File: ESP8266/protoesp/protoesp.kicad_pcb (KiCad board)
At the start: 2 copper layers, 97.5 x 90 mm, 192 parts, among them CN1 EPINS_TOP, CN10 USB_CURSED, CN11 CH_SPI, CN12 CH_I2C, CN13 CH341_PROG, CN14 CH_PROG, CN2 EPINS_BOTTOM, CN20 BATT, CN3 ESP_PROG, CN30 BUTTON_CONN, CN31 LDR_CONN, CN32 RGB_CONN, CN33 595_CONN, CN34 595_OUTS, CN35 595CHAIN_CONN, CN36 E_I2C, CN37 E_SPI, CN38 DRV_CONN, J1 0R, J11 0R, J17 0R, J19 0R, J2 0R, J22 0R, J7 0R, J8 0R, J9 0R, P1 PROTO_SPACE, Q1 BC817, Q2 CJ2305, SW1 RST, SW2 BUTTON, U1 CH341, U2 AP1117-33, U3 LTH7R, U4 74HC595, U5 AP2112K-3.3, U6 ESP32-WROOM-32, Y1 12MHz

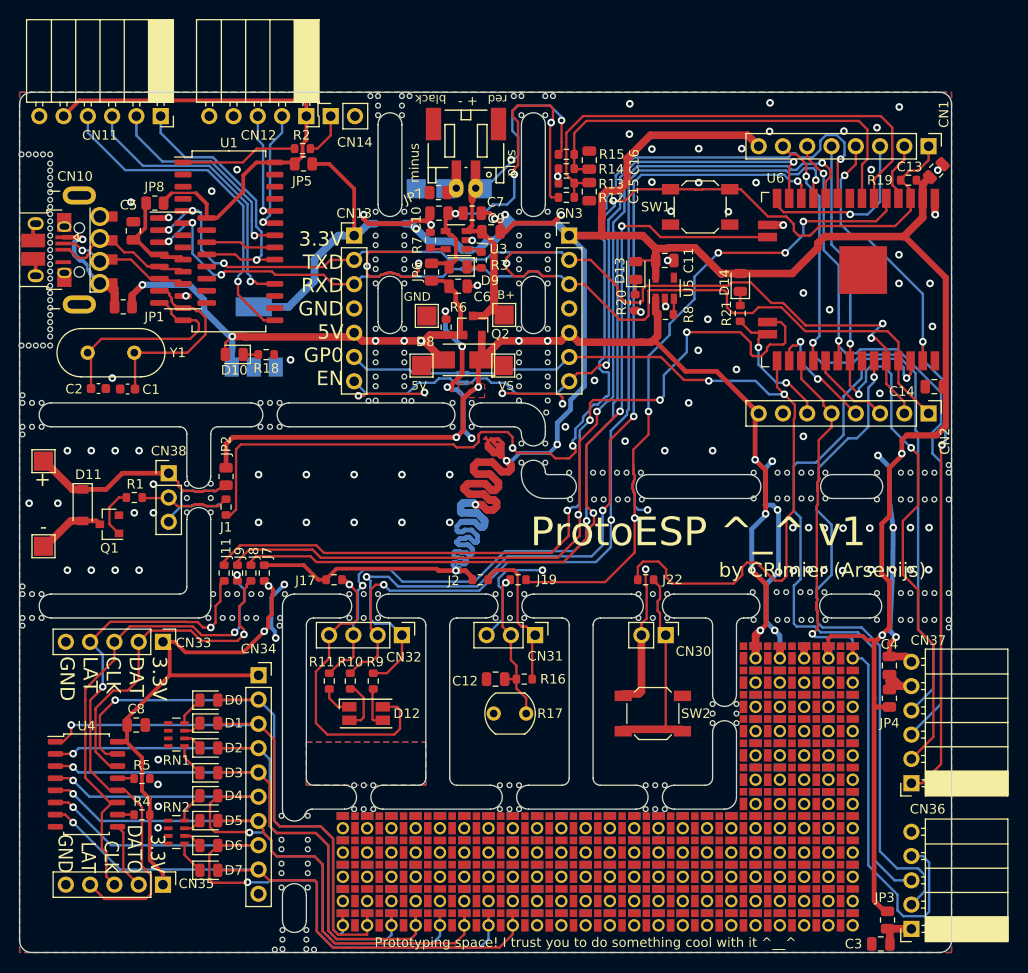
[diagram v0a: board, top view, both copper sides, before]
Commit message: Final changes - only small silk art things left before I'll order it, otherwise, this is orderable!
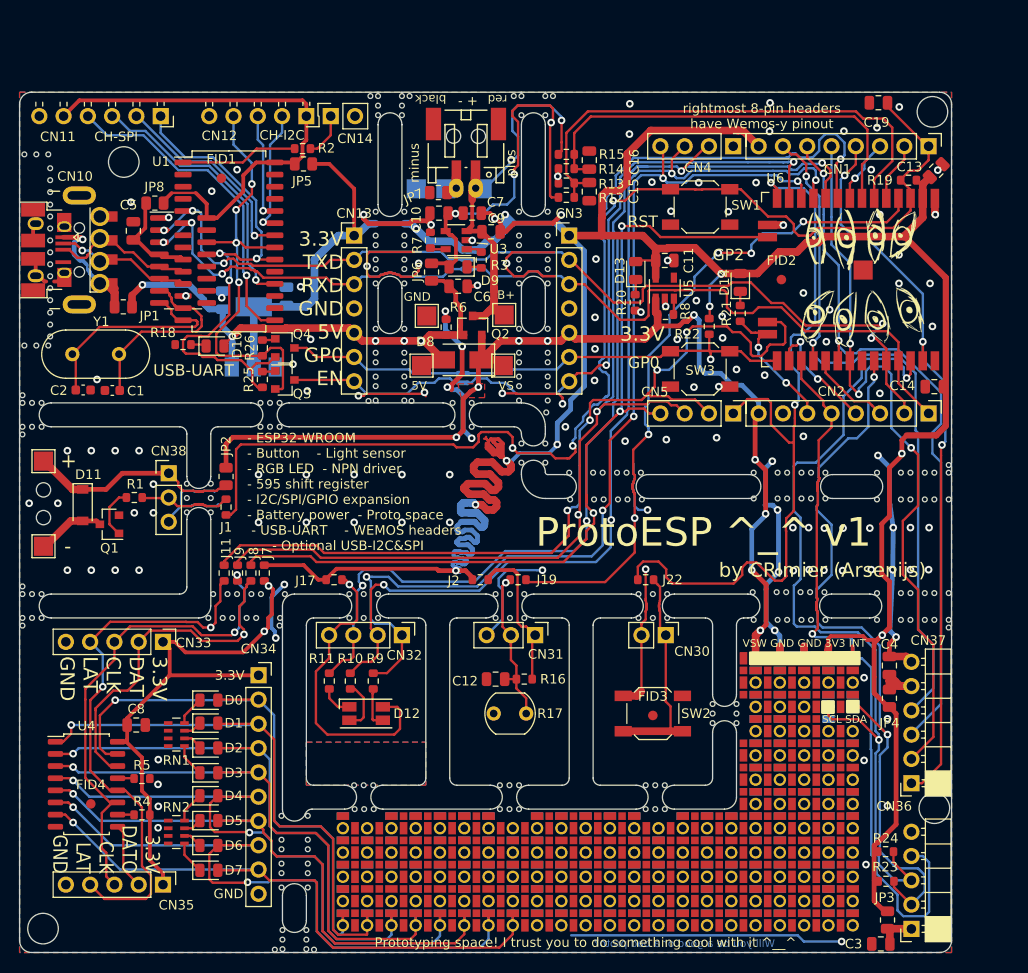
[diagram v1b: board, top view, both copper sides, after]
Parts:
- added C17: 100nF, Capacitor_SMD:C_0805_2012Metric, B.Cu at (71.2, 71.8)
- added C18: 100nF, Capacitor_SMD:C_0805_2012Metric, B.Cu at (77.9, 71.3)
- added C19: 100nF, Capacitor_SMD:C_0805_2012Metric, F.Cu at (139.8, 51.1)
- added CN4: EPINS_TOP_E, Connector_PinHeader_2.54mm:PinHeader_1x04_P2.54mm_Vertical, F.Cu at (124.7, 55.6)
- added CN5: EPINS_BOTTOM_E, Connector_PinHeader_2.54mm:PinHeader_1x04_P2.54mm_Vertical, F.Cu at (124.7, 83.6)
- added FID1: Fiducial, Fiducial:Fiducial_1mm_Mask2mm, F.Cu at (71.1, 59.0)
- added FID2: Fiducial, Fiducial:Fiducial_1mm_Mask2mm, F.Cu at (129.7, 69.6)
- added FID3: Fiducial, Fiducial:Fiducial_1mm_Mask2mm, F.Cu at (116.2, 115.2)
- added FID4: Fiducial, Fiducial:Fiducial_1mm_Mask2mm, F.Cu at (57.5, 124.5)
- added G***: LOGO, protoesp:ey, F.Cu at (138.2, 69.4)
- added H1: MountingHole, MountingHole:MountingHole_3.2mm_M3, F.Cu at (60.9, 57.3)
- added H1: pin_hole, protoesp:PinHole_1,5mm, F.Cu at (52.5, 91.6)
- added H1: pin_hole, protoesp:PinHole_1,5mm, F.Cu at (52.5, 94.5)
- added H1: pin_hole, protoesp:PinHole_1,5mm, F.Cu at (98.0, 54.6)
- added H1: pin_hole, protoesp:PinHole_1,5mm, F.Cu at (95.4, 54.6)
- added H2: MountingHole, MountingHole:MountingHole_3.2mm_M3, F.Cu at (52.5, 137.5)
- added H3: MountingHole, MountingHole:MountingHole_3.2mm_M3, F.Cu at (145.5, 52.0)
- added H4: MountingHole, MountingHole:MountingHole_3.2mm_M3, F.Cu at (145.7, 124.9)
- added Q3: BC817, Package_TO_SOT_SMD:SOT-23, F.Cu at (77.8, 80.1)
- added Q4: BC817, Package_TO_SOT_SMD:SOT-23, F.Cu at (77.8, 76.8)
- added R22: 4K7, Resistor_SMD:R_0603_1608Metric, F.Cu at (122.2, 74.5)
- added R23: 1K8, Resistor_SMD:R_0603_1608Metric, F.Cu at (140.7, 132.6)
- added R24: 1K8, Resistor_SMD:R_0603_1608Metric, F.Cu at (140.6, 129.4)
- added R25: 4K7, Resistor_SMD:R_0603_1608Metric, F.Cu at (75.4, 80.0)
- added R26: 4K7, Resistor_SMD:R_0603_1608Metric, F.Cu at (75.4, 76.8)
- added SW3: GP0, Button_Switch_SMD:SW_SPST_SKQG_WithStem, F.Cu at (121.2, 79.0)
- SW1: value RST -> EN
- TP7: value B+ -> B-
- moved R18 8.76 mm to (67.1, 76.4), turned to 0 degrees
- moved REF** 2.70 mm to (50.5, 76.5), turned to 0 degrees
- moved REF** 2.70 mm to (50.5, 56.5), turned to 0 degrees
- moved D10 2.19 mm to (70.5, 76.5), turned to 0 degrees
- moved C2 1.61 mm to (56.6, 81.2)
- moved Y1 1.61 mm to (60.4, 77.4)
- moved C1 1.61 mm to (59.7, 81.2)
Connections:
- net CH_RST renamed CH_EN
- net Net-(CN38-Pad1) renamed DRV+
- net Net-(D11-Pad2) renamed DRV-
- CN1 pad 2: POT -> IO39
- CN1 pad 3: IO12 -> IO32
- CN12 pad 4: Net-(CN12-Pad4) -> CH_~RTS
- CN3 pad 6: BUTTON -> E_GP0
- NT6 pad 2: BUTTON -> E_GP0
- U6 pad 14: IO12 -> BUTTON
- U6 pad 25: BUTTON -> E_GP0
- U6 pad 4: POT -> LIGHT
- U6 pad 5: LIGHT -> IO39
- U6 pad 8: Net-(U6-Pad8) -> IO32
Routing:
- net CH_~RTS: track 7.35 -> 47.0 mm, vias 0 -> 4
- net E_GP0: track 0.00 -> 36.4 mm, vias 0 -> 1
- net GND: track 197.0 -> 227.6 mm, vias 118 -> 134
- net CH_MOSI: track 28.8 -> 56.9 mm, vias 1 -> 3
- net IO12: track 18.3 -> 0.00 mm, vias 1 -> 0
- net +3V3: track 336.4 -> 353.8 mm, vias 8 -> 10
- net E_SCL: track 76.5 -> 87.8 mm, vias 1 -> 2
- net 595_CLK: track 100.8 -> 110.9 mm
- net E_SDA: track 70.4 -> 79.1 mm, vias 1 -> 2
- net LED_RED: track 104.8 -> 113.1 mm, vias 3 -> 4
- net 595_LAT: track 85.8 -> 93.1 mm
- net IO32: track 0.00 -> 6.76 mm, vias 0 -> 1
- net CH_GP0: track 11.6 -> 18.2 mm
- net E_EN: track 78.9 -> 85.3 mm
- net CH_EN: track 12.3 -> 18.6 mm
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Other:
- board text added: "+"
- board text added: "-"
- board text added: "- ESP32-WROOM - Button - Light sensor - RGB LED - NPN driver - 595 shift register - I2C/SPI/GPIO expansion - Battery power - Proto space - USB-UART - WEMOS headers - Optional USB-I2C&SPI"
- board text added: "23 19 18 17"
- board text added: "3.3V"
- board text added: "CH-I2C"
- board text added: "CH-SPI"
- board text added: "CH340/1"
- board text added: "CMOSI CMISO CCLK CCS CVCC GND"
- board text added: "EN G39 G12 G23 G19 G18 G17 GND 3.3V G25 G26 G27"
- board text added: "ESP32"
- board text added: "GND 3.3V CS SCK SO SI"
- board text added: "GND ACT CVCC CSDA CSCL NC GND"
- board text added: "GND INT SCL SDA 3.3V"
- board text added: "GP12"
- board text added: "GP2"
- board text added: "GP21 22 16"
- board text added: "GP36"
- board text added: "I2C/GPIO header"
- board text added: "INT 3V3 GND GND VSW"
- board text added: "Part of the FANGY project."
- board text added: "ProtoESP ESP32 PCB v1"
- board text added: "ProtoESP protoSpace PCB v1"
- board text added: "RST"
- board text added: "SCL SDA"
- board text added: "SPI/GPIO header"
- board text added: "TXD RXD G5 G4 G16 G2 GND VSW G0 G15 G14 G13"
- board text added: "This PCB houses an ESP32 and a family of fun things for your learning, leisure and helpful purposes. I hope that this PCB becomes your friend. -A"
- board text added: "USB-UART"
- board text added: "VSW = 3.5V-5V"
- board text added: "VSW GND GND 3V3 INT"
- board text added: "Will you be a good or a bad proto?"
- board text added: "batt ery input"
- board text added: "rightmost 8-pin headers have Wemos-y pinout"
- board text added: "spaaaaace"
- board text removed: "GND ACT CVCC CSDA CSCL NC GND CMOSI CMISO CCLK CCS CVCC GND"
- board text removed: "GP0"
- board text removed: "GP35"
- board text removed: "bat tery in put"
